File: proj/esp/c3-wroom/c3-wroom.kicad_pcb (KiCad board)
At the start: 2 copper layers, 20.8 x 37.8 mm, 15 parts, among them J1 USB_C_Receptacle_USB2.0_16P, J2 OUT1, J3 OUT2, SW1 SW_BOOT, SW2 SW_BOOT, U1 ESP32-C3-WROOM-02, U2 AP7333

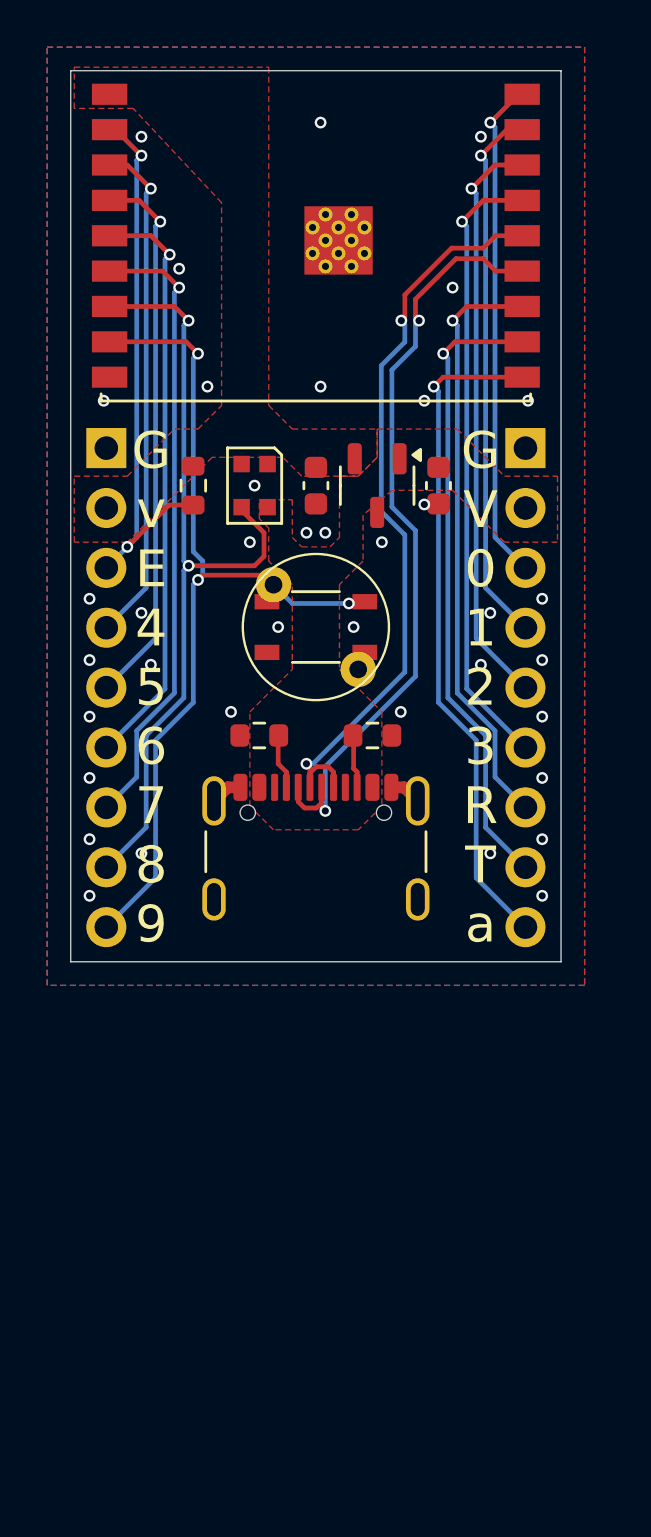
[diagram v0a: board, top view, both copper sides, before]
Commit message: -
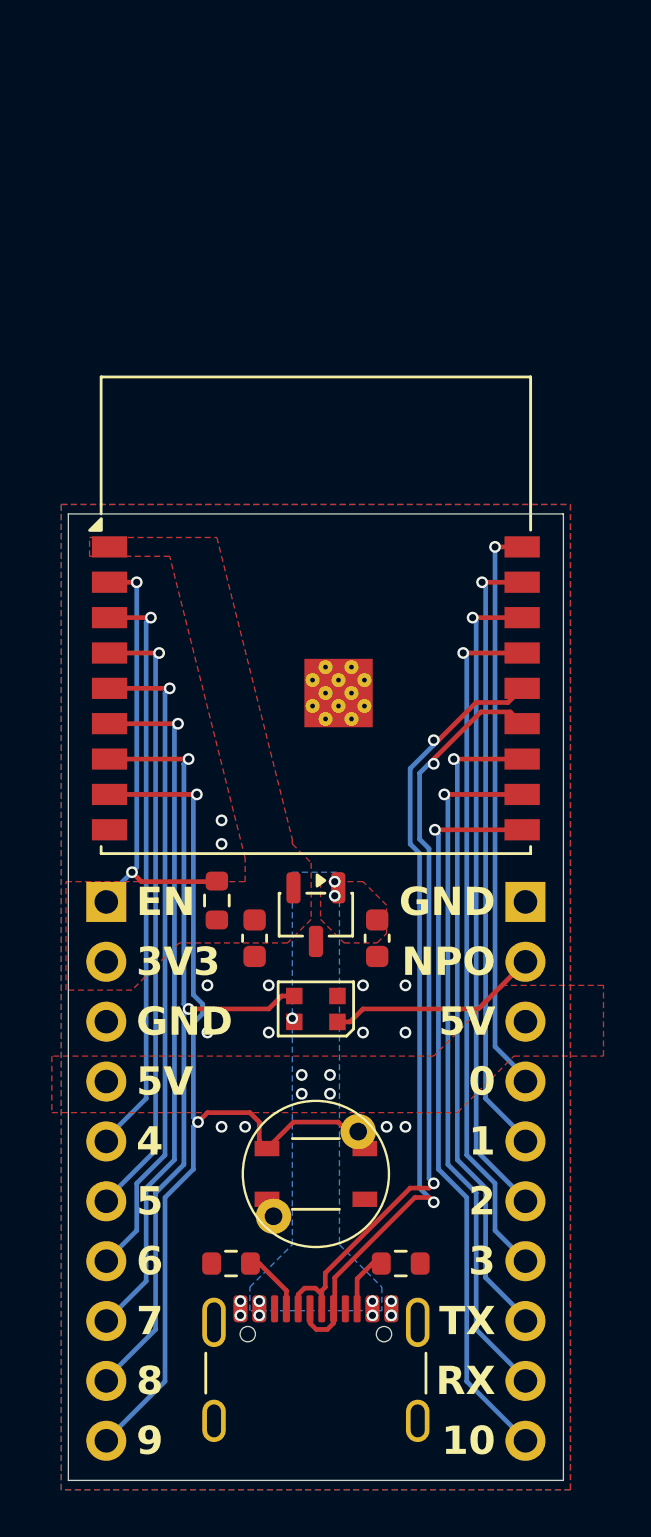
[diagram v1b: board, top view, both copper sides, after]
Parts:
- removed G***: LOGO, LOGO
- added ?: LOGO, Library:mcbeeringi_icon_10mm, B.Cu at (100.0, 85.6)
- J2, J3: footprint Connector_PinHeader_2.54mm:PinHeader_1x09_P2.54mm_Vertical -> Connector_PinHeader_2.54mm:PinHeader_1x10_P2.54mm_Vertical
- R2, R3: value 5.1k -> 4k7
- moved SW1 23.2 mm to (100.0, 109.0), turned to -135 degrees
- moved SW2 23.2 mm to (100.0, 109.0)
- moved R2 22.4 mm to (96.4, 112.8)
- moved R3 22.4 mm to (103.6, 112.8)
- moved D1 22.4 mm to (100.0, 102.0), turned to 180 degrees
- moved J1 22.1 mm to (100.0, 118.4)
- moved C1 19.4 mm to (102.6, 99.0)
- moved C2 19.4 mm to (97.4, 99.0)
- moved J2 19.2 mm to (91.1, 97.5)
- moved J3 19.2 mm to (108.9, 97.5)
- moved U1 19.2 mm to (100.0, 88.4)
- moved U2 18.4 mm to (100.0, 98.0)
- moved R1 17.6 mm to (95.8, 97.4), turned to 90 degrees
- moved ? 17.2 mm to (100.0, 93.2), turned to -90 degrees
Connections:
- D1 pad 1: unconnected-(D1-DOUT-Pad1) -> NP_OUT
- J2 pad 1: GND -> EN
- J2 pad 3: EN -> GND
- J2 pad 4: IO4 -> VBUS
- J2 pad 5: IO5 -> IO4
- J2 pad 6: IO6 -> IO5
- J2 pad 7: IO7 -> IO6
- J2 pad 8: IO8 -> IO7
- J2 pad 9: IO9 -> IO8
- J3 pad 2: VBUS -> NP_OUT
- J3 pad 3: IO0 -> VBUS
- J3 pad 4: IO1 -> IO0
- J3 pad 5: IO2 -> IO1
- J3 pad 6: IO3 -> IO2
- J3 pad 7: TXD -> IO3
- J3 pad 8: RXD -> TXD
- J3 pad 9: IO10 -> RXD
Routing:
- net NP_OUT: track 0.00 -> 9.03 mm
- net IO9: track 37.2 -> 42.5 mm, vias 3 -> 2
- net EN: track 23.6 -> 19.0 mm
- net IO4: track 21.6 -> 24.8 mm
- net IO1: track 23.0 -> 26.2 mm
- net IO2: track 24.7 -> 27.8 mm
- net IO6: track 24.9 -> 28.0 mm
- net IO3: track 26.3 -> 29.4 mm
- net IO5: track 23.2 -> 26.3 mm
- net IO0: track 21.4 -> 24.4 mm
- net IO7: track 26.6 -> 29.5 mm
- net TXD: track 25.1 -> 28.0 mm
- net RXD: track 26.8 -> 29.6 mm
- net GND: track 2.72 -> 0.00 mm, vias 38 -> 18
- net IO10: track 28.5 -> 31.2 mm
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- added copper zone on B.Cu, net VBUS
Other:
- board size 20.8 x 37.8 mm -> 21 x 41 mm
- board text added: "0"
- board text added: "1"
- board text added: "10"
- board text added: "10k"
- board text added: "1u"
- board text added: "2"
- board text added: "3"
- board text added: "3V3"
- board text added: "4"
- board text added: "4k7"
- board text added: "5"
- board text added: "5V"
- board text added: "6"
- board text added: "7"
- board text added: "8"
- board text added: "9"
- board text added: "@McbeEringi"
- board text added: "ALPS"
- board text added: "AP7333"
- board text added: "EN"
- board text added: "ESP32-C3 dev-board"
- board text added: "GND"
- board text added: "NPO"
- board text added: "RX"
- board text added: "SKRP SKRG"
- board text added: "TX"
- board text added: "WS2812-2020"
- board text removed: "ESP32 C3 dev board"
- board text removed: "ESP32-C3 WROOM-02"
- board text removed: "G V 0 1 2 3 R T a"
- board text removed: "G v E 4 5 6 7 8 9"
